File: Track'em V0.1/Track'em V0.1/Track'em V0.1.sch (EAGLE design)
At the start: 34 parts, among them IC1 SAM-M8Q, J1 CORTEX_DEBUG_PTH, U2 3.3V/150mA

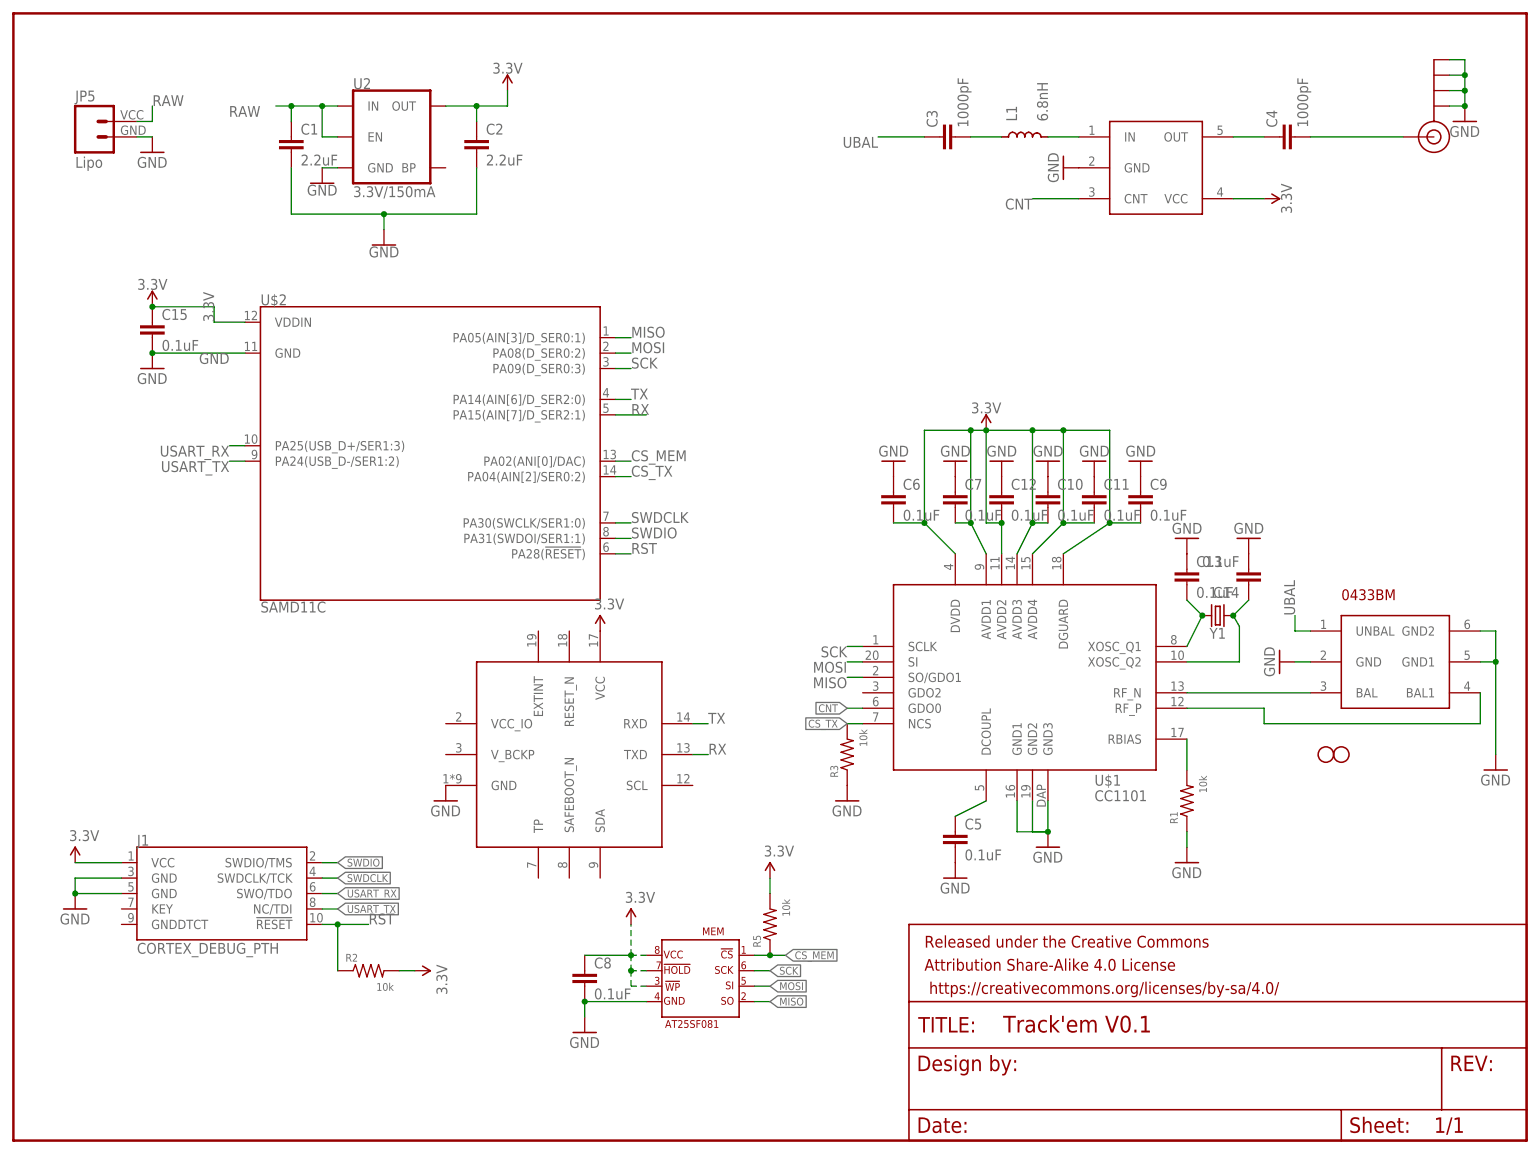
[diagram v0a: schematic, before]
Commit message: track'em updates
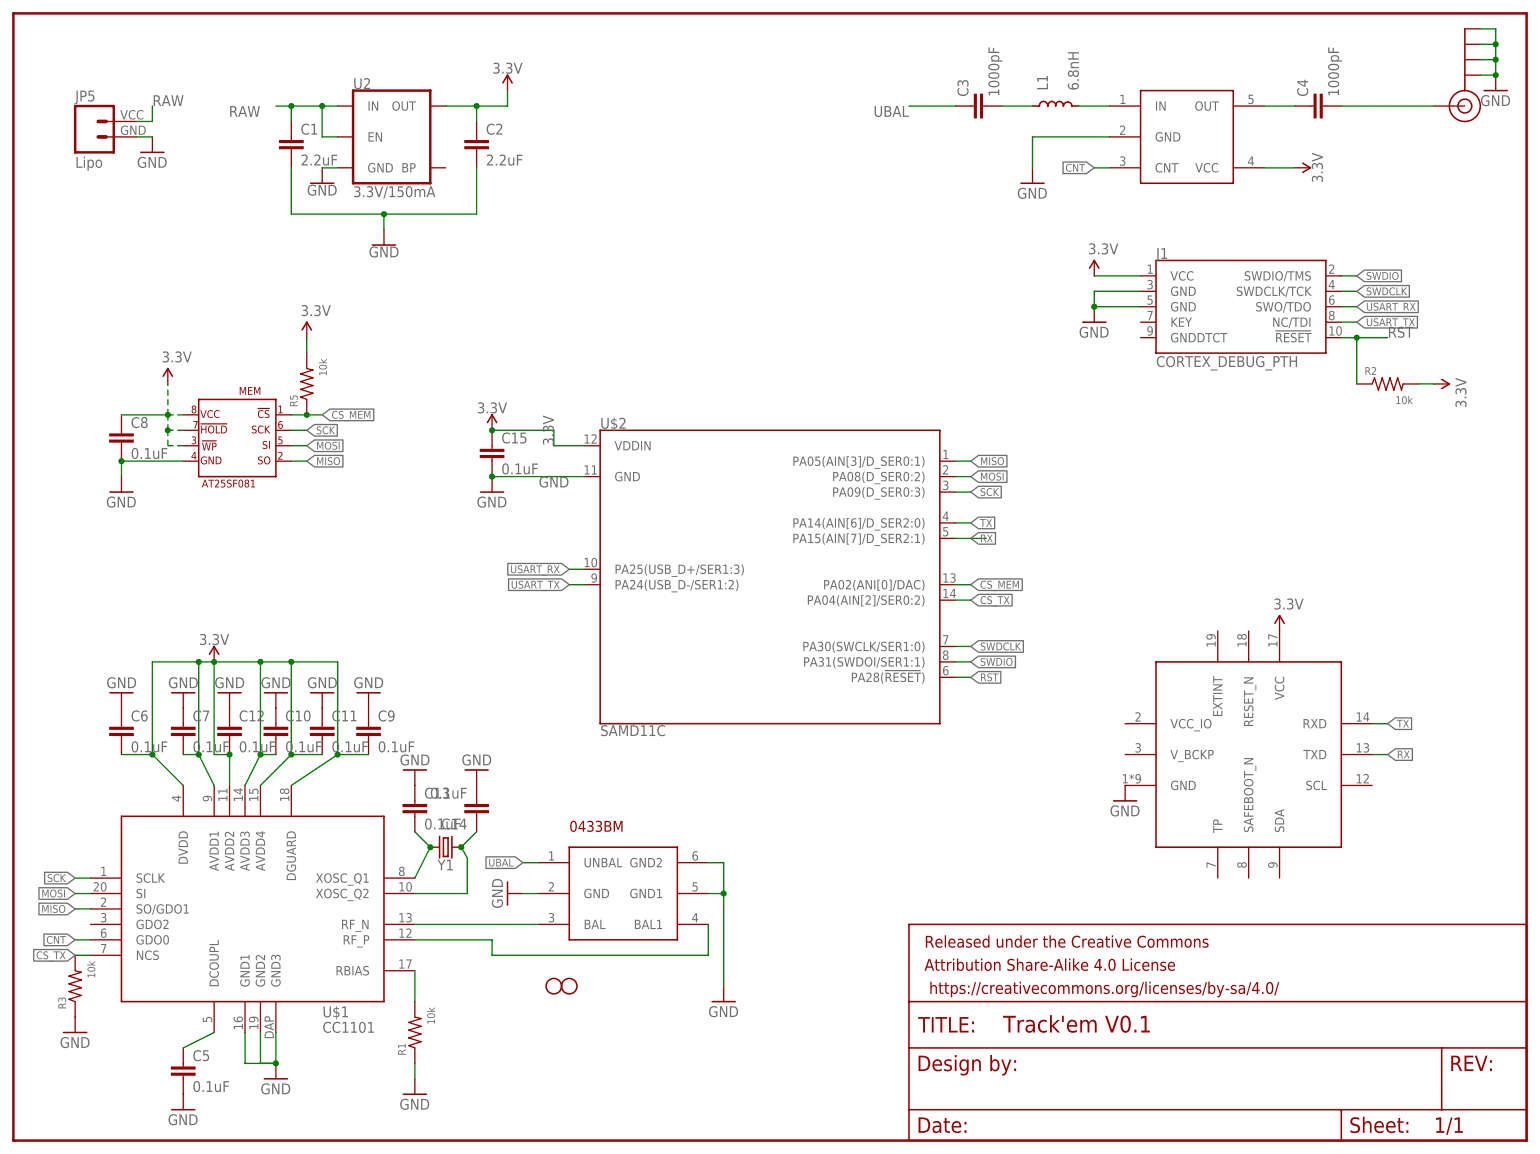
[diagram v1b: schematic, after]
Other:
- moved on the sheet: C10, C11, C12, C13, C14, C15, C3, C4, C5, C6, C7, C8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
